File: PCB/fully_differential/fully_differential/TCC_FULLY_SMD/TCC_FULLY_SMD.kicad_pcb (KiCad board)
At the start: 2 copper layers, 48 parts, among them IC1 THP210DR, IC2 THP210DR, J1 Conn_01x03, J10 Conn_01x02, J11 Conn_01x02, J2 Conn_01x03, J3 Conn_01x02, J4 Conn_01x02, J5 Conn_01x02, J6 Conn_01x02, J7 Conn_01x02, J8 Conn_01x02, U1 L7805, U2 TL072, U3 TL072, U4 L7809, U5 L7909, U6 TL072, U7 TL072

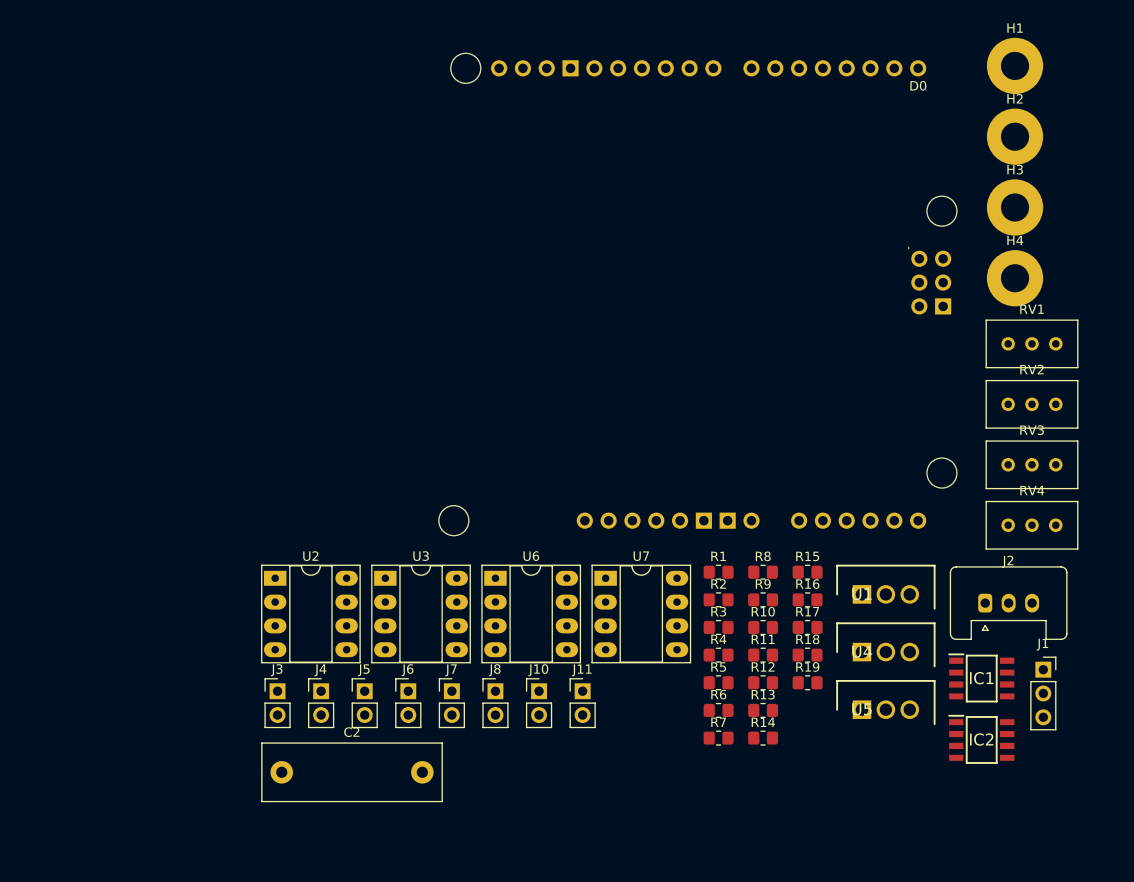
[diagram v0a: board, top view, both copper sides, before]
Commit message: schamatic
init
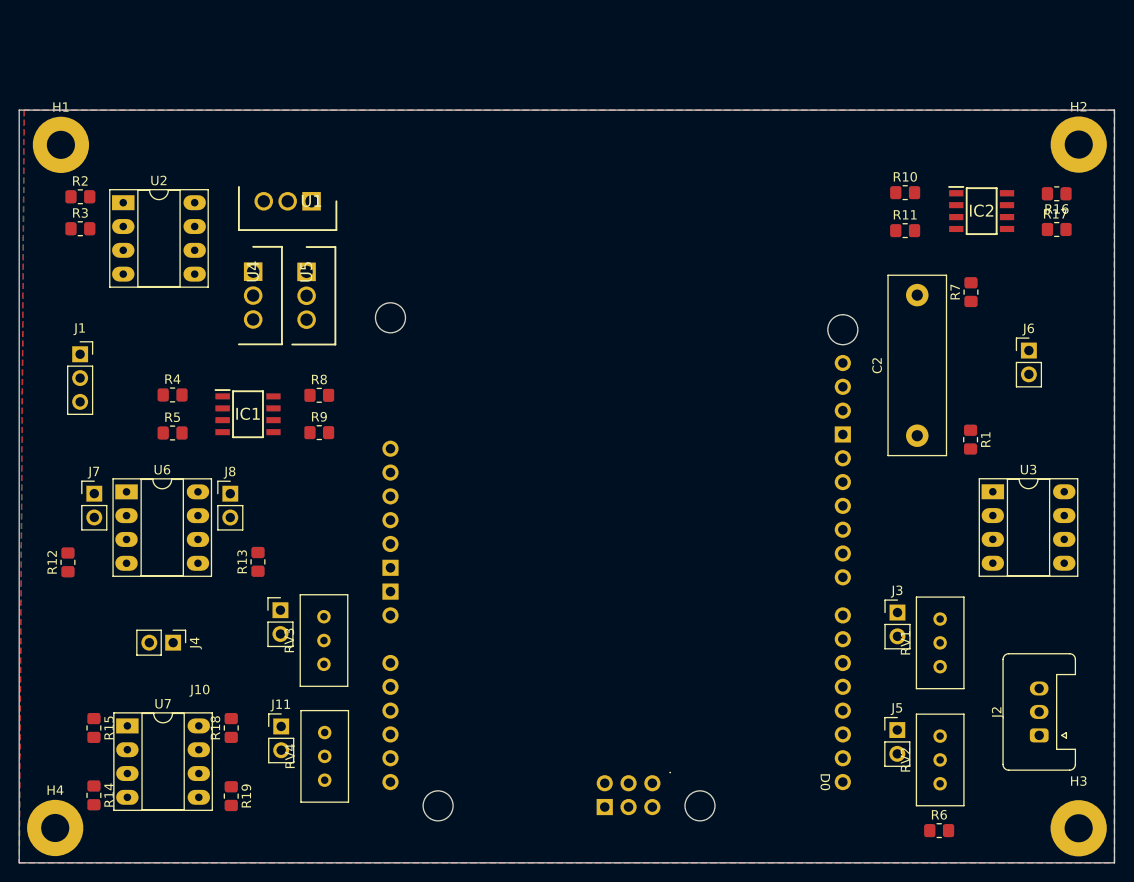
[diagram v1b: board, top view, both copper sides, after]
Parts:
- moved H4 118.0 mm to (92.7, 133.7)
- moved J1 108.1 mm to (95.4, 83.2)
- moved H1 102.1 mm to (93.3, 60.9)
- moved IC1 83.2 mm to (113.3, 89.6)
- moved RV4 81.1 mm to (121.5, 123.5), turned to 90 degrees
- moved R2 80.5 mm to (95.4, 66.4)
- moved R3 80.3 mm to (95.4, 69.8)
- moved RV3 79.7 mm to (121.4, 111.2), turned to 90 degrees
- moved R15 77.9 mm to (96.8, 123.1), turned to -90 degrees
- moved C2 76.7 mm to (184.7, 91.9), turned to 90 degrees
- moved U4 76.6 mm to (113.8, 74.4), turned to -90 degrees
- moved J6 75.5 mm to (196.6, 82.8)
- moved U5 75.4 mm to (119.5, 74.4), turned to -90 degrees
- moved R12 75.3 mm to (94.1, 105.4), turned to 90 degrees
- moved U1 72.2 mm to (120.0, 66.9), turned to 180 degrees
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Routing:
- added copper zone on B.Cu, net GND
- added copper zone on F.Cu, net GND
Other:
- board outline added: 116.9 x 80.3 mm
